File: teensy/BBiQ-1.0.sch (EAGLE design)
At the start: 29 parts, among them IC1 ESP-WROOM-02, J1 MJ-2506N, J2 MJ-2506N, J3 MJ-2506N, J4 MJ-2506N, T1 2N3904

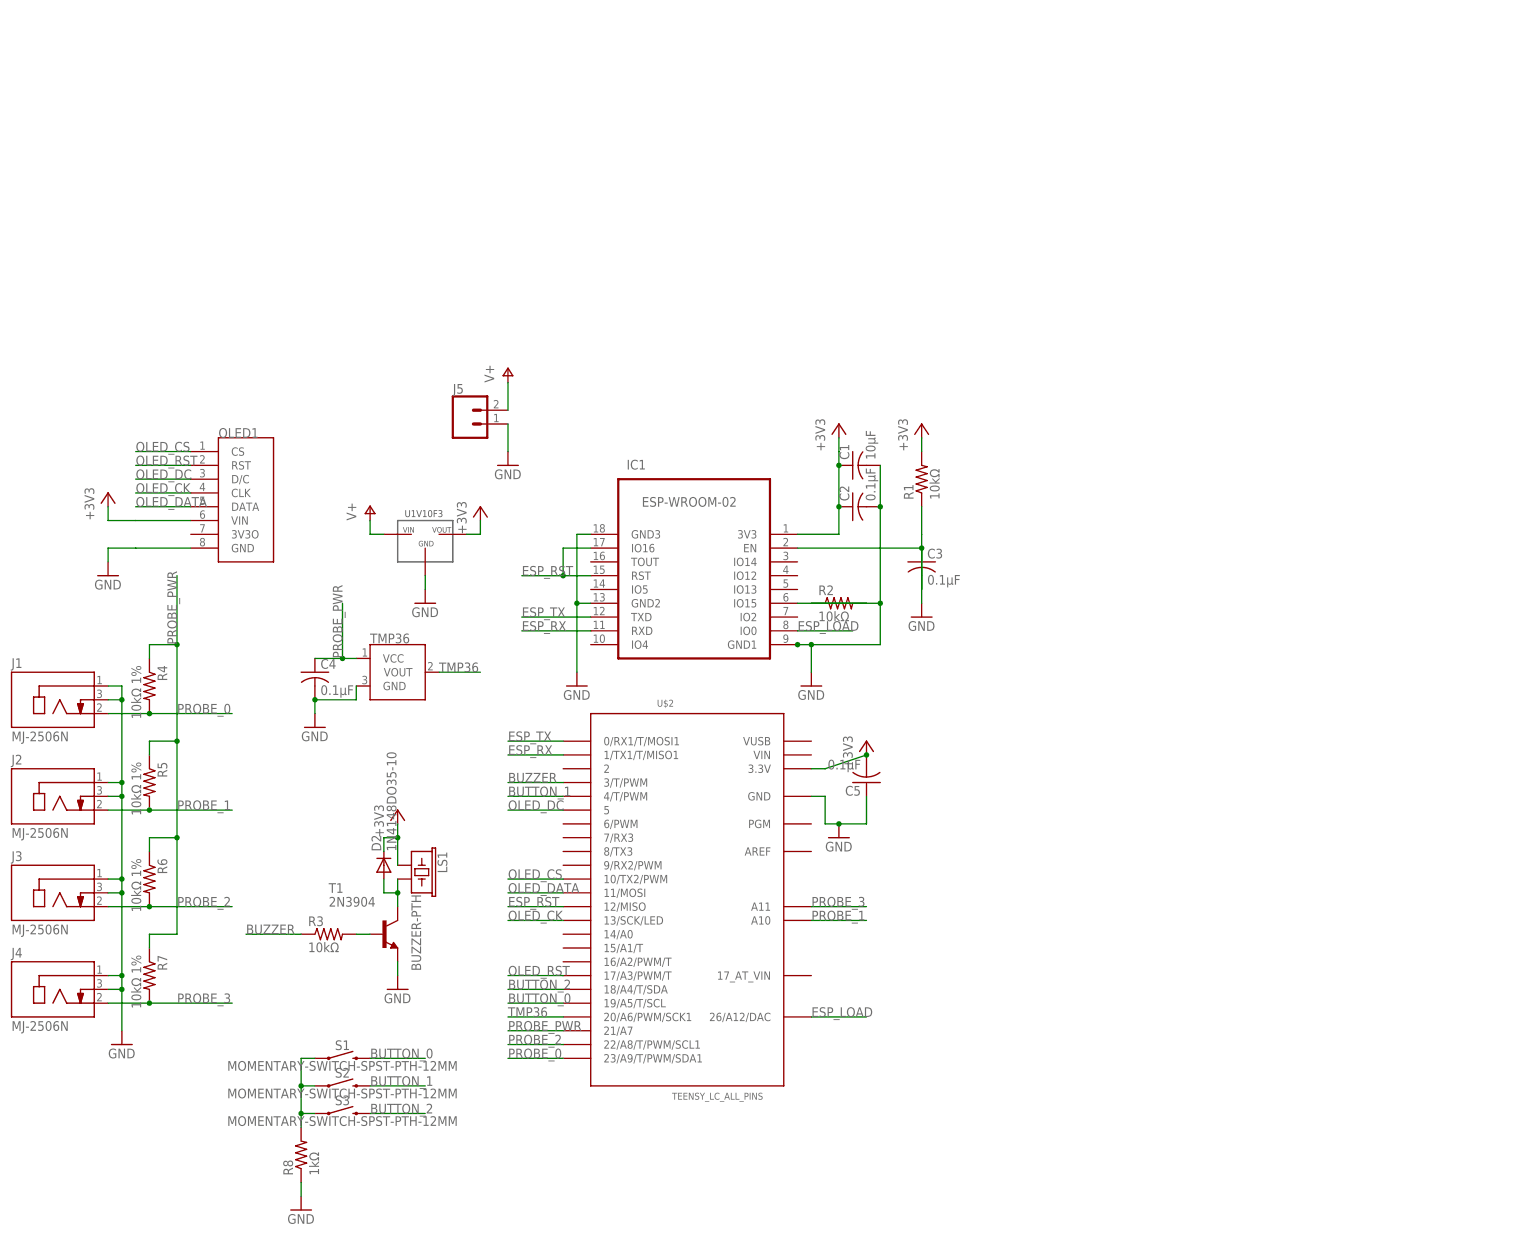
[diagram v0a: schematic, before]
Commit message: New projects for final TeensyLC/ESP-WROOM-02 code
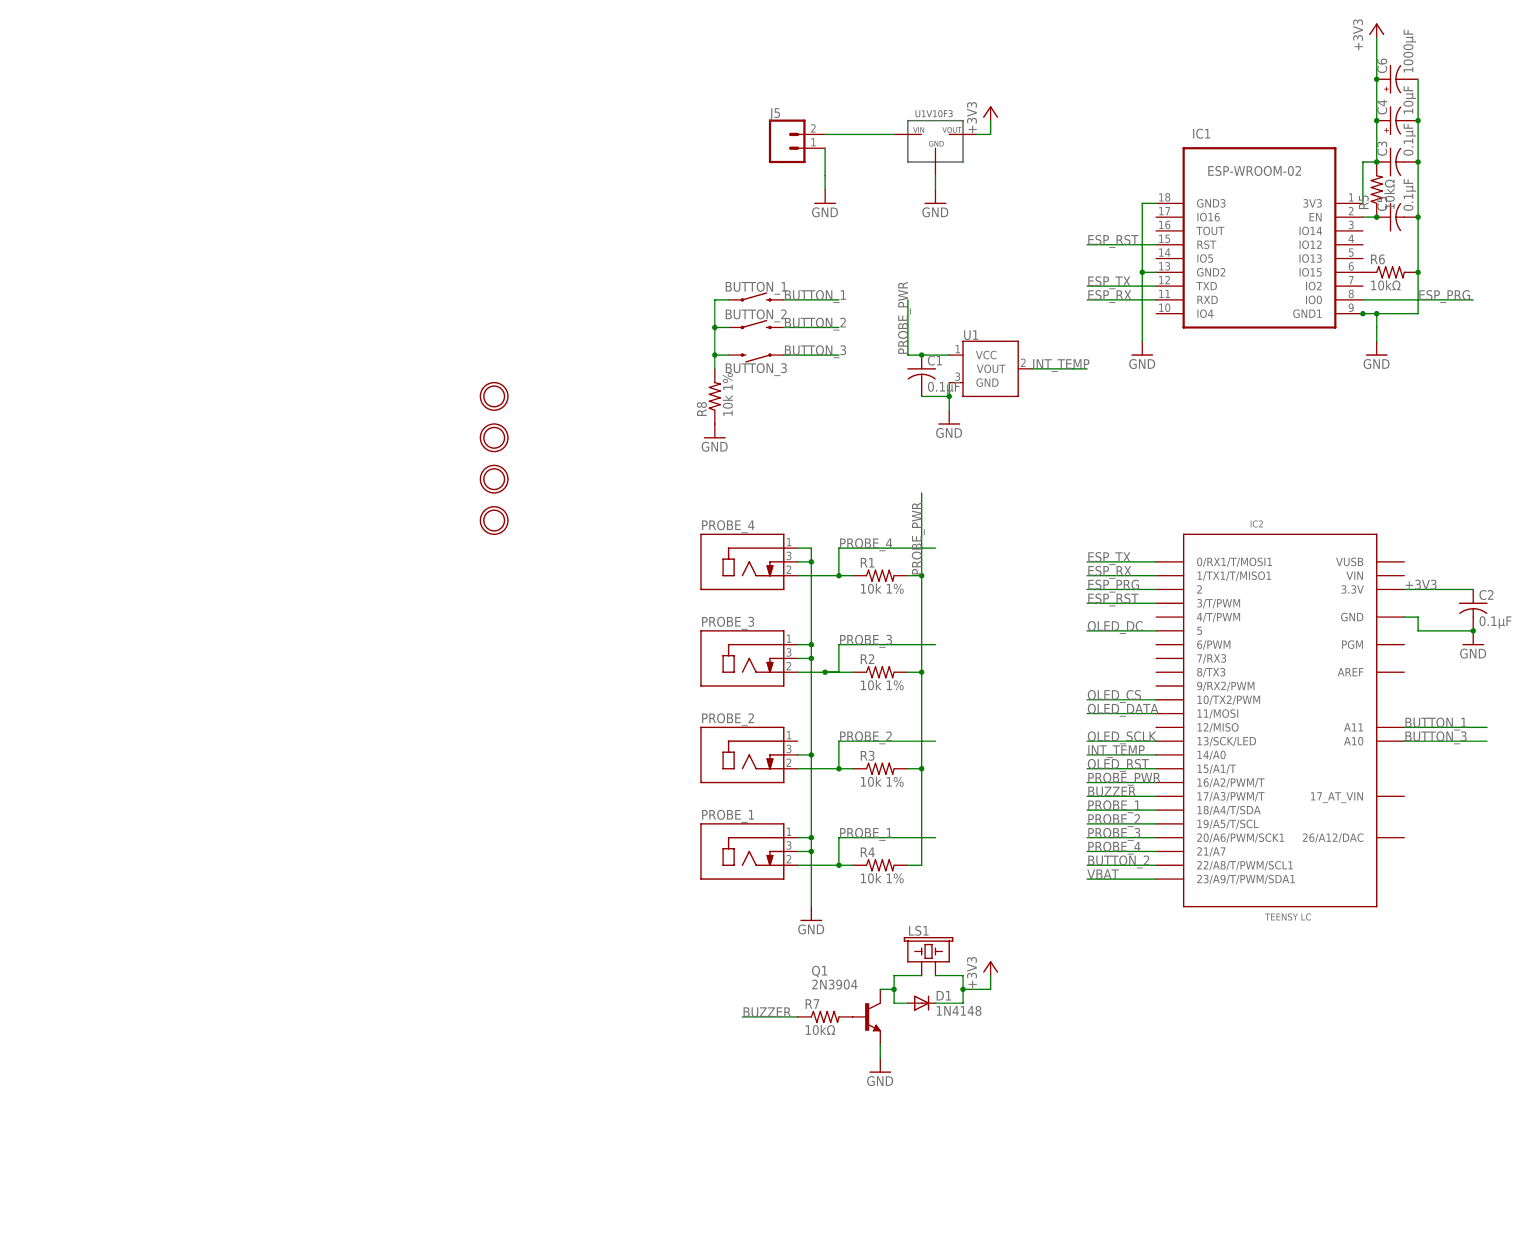
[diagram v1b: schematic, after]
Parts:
- removed D2: 1N4148DO35-10, diode:1N4148DO35-10
- removed J1, J2, J3, J4: MJ-2506N, MJ-2506N:MJ-2506N
- removed OLED1: ADAFRUIT_128X32_SPI_OLED, Adafruit OLED 128x32 Mono:ADAFRUIT_128X32_SPI_OLED
- removed S1, S2, S3: MOMENTARY-SWITCH-SPST-PTH-12MM, SparkFun-Switches:MOMENTARY-SWITCH-SPST-PTH-12MM
- removed T1: 2N3904, transistor:2N3904
- removed TMP36: (no value), SparkFun-Sensors:TMP36GT9
- removed U$1: U1V10F3, U1V10F3:U1V10F3
- added BUTTON_1, BUTTON_2, BUTTON_3: MOMENTARY-SWITCH-SPST-PTH-6.0MM, SparkFun-Switches:MOMENTARY-SWITCH-SPST-PTH-6.0MM
- added C6: 1000µF, resistor:CPOL-USE3.5-8
- added D1: 1N4148, diode:1N4148DO35-7
- added IC2: TEENSY LC, Teensy_3_and_LC_Series_Boards_v1.4:TEENSY_LC_ALL_PINS
- added PROBE_1, PROBE_2, PROBE_3, PROBE_4: MJ-2506N, MJ-2506N:MJ-2506N
- added Q1: 2N3904, transistor:2N3904
- added U$3, U$4, U$5, U$6: MOUNTINGHOLE2.5, microbuilder:MOUNTINGHOLE2.5
- added U1: (no value), SparkFun-Sensors:TMP36GT9
- C1: value 10µF -> 0.1µF
- C4: value 0.1µF -> 10µF; device resistor:C-US025-025X050 -> resistor:CPOL-USE2-5
- R1, R2, R3: value 10kΩ -> 10k 1%; device resistor:R-US_0204/5 -> resistor:R-US_0207/7
- R4: value 10kΩ 1% -> 10k 1%; device resistor:R-US_0204/5 -> resistor:R-US_0207/7
- R5, R6, R7: value 10kΩ 1% -> 10kΩ; device resistor:R-US_0204/5 -> resistor:R-US_0207/7
- R8: value 1kΩ -> 10k 1%; device resistor:R-US_0204/5 -> resistor:R-US_0207/7
- U$2: value TEENSY_LC_ALL_PINS -> U1V10F3; device Teensy_3_and_LC_Series_Boards_v1.4:TEENSY_LC_ALL_PINS -> U1V10F3:U1V10F3
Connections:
- removed net BUTTON_0: S1.2, U$2.19/A5/T/SCL
- removed net ESP_LOAD: IC1.IO0, U$2.26/A12/DAC
- removed net N$6: D2.A, LS1.2, T1.C
- removed net N$7: R8.2, S1.1, S2.1, S3.1
- removed net OLED_CK: OLED1.CLK, U$2.13/SCK/LED
- removed net PROBE_0: J1.2, R4.2, U$2.23/A9/T/PWM/SDA1
- removed net TMP36: TMP36.VOUT, U$2.20/A6/PWM/SCK1
- new net BUTTON_3: BUTTON_3.1, IC2.A10
- new net ESP_EN: C5.1, IC1.EN, R5.1
- new net ESP_PRG: IC1.IO0, IC2.2
- new net INT_TEMP: IC2.14/A0, U1.VOUT
- new net N$1: IC1.IO15, R6.1
- new net OLED_SCLK: IC2.13/SCK/LED
- new net PROBE_4: IC2.21/A7, PROBE_4.2, R1.1
- net +3V3: now also C3.1, C4.+, C6.+, D1.C, IC2.3.3V, LS1.2, R5.2, U$2.VOUT; no longer C1.1, C5.2, D2.C, LS1.1, OLED1.VIN, R1.2, U$1.VOUT, U$2.3.3V
- net BUTTON_1: now also BUTTON_1.2, IC2.A11; no longer S2.2, U$2.4/T/PWM
- net BUTTON_2: now also BUTTON_2.2, IC2.22/A8/T/PWM/SCL1; no longer S3.2, U$2.18/A4/T/SDA
- net BUZZER: now also IC2.17/A3/PWM/T, R7.1; no longer R3.1, U$2.3/T/PWM
- net ESP_RST: now also IC2.3/T/PWM; no longer IC1.IO16, U$2.12/MISO
- net ESP_RX: now also IC2.1/TX1/T/MISO1; no longer U$2.1/TX1/T/MISO1
- net ESP_TX: now also IC2.0/RX1/T/MOSI1; no longer U$2.0/RX1/T/MOSI1
- net GND: now also C3.2, C4.-, C5.2, C6.-, IC2.GND, PROBE_1.1, PROBE_1.3, PROBE_2.3, PROBE_3.1, PROBE_3.3, PROBE_4.1, PROBE_4.3, Q1.E, R6.2, U1.GND; no longer C3.1, C4.2, C5.1, J1.1, J1.3, J2.1, J2.3, J3.1, J3.3, J4.1, J4.3, OLED1.GND, R2.1, T1.E, TMP36.GND, U$1.GND
- net N$2: now also Q1.B, R7.2; no longer C3.2, IC1.EN, R1.1
- net N$3: now also D1.A, LS1.1, Q1.C; no longer IC1.IO15, R2.2
- net N$4: now also BUTTON_1.1, BUTTON_2.1, BUTTON_3.2, R8.2; no longer R3.2, T1.B
- net OLED_CS: now also IC2.10/TX2/PWM; no longer OLED1.CS, U$2.10/TX2/PWM
- net OLED_DATA: now also IC2.11/MOSI; no longer OLED1.DATA, U$2.11/MOSI
- net OLED_DC: now also IC2.5; no longer OLED1.D/C, U$2.5
- net OLED_RST: now also IC2.15/A1/T; no longer OLED1.RST, U$2.17/A3/PWM/T
- net PROBE_1: now also IC2.18/A4/T/SDA, PROBE_1.2, R4.1; no longer J2.2, R5.2, U$2.A10
- net PROBE_2: now also IC2.19/A5/T/SCL, PROBE_2.2, R3.1; no longer J3.2, R6.2, U$2.22/A8/T/PWM/SCL1
- net PROBE_3: now also IC2.20/A6/PWM/SCK1, PROBE_3.2, R2.1; no longer J4.2, R7.2, U$2.A11
- net PROBE_PWR: now also C1.1, IC2.16/A2/PWM/T, R1.2, R2.2, R3.2, R4.2, U1.VCC; no longer C4.1, R4.1, R5.1, R6.1, R7.1, TMP36.VCC, U$2.21/A7
- net VBAT: now also IC2.23/A9/T/PWM/SDA1, U$2.VIN; no longer U$1.VIN
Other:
- moved on the sheet: C1, C2, C3, C5, IC1, J5, LS1, R1, R2, R3, R4, R5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
